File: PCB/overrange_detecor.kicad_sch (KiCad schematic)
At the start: 25 parts, among them Q301 DMP3125L, Q302 DMP3125L, U301 TLV3542, U302 74HC00, U303 LM321

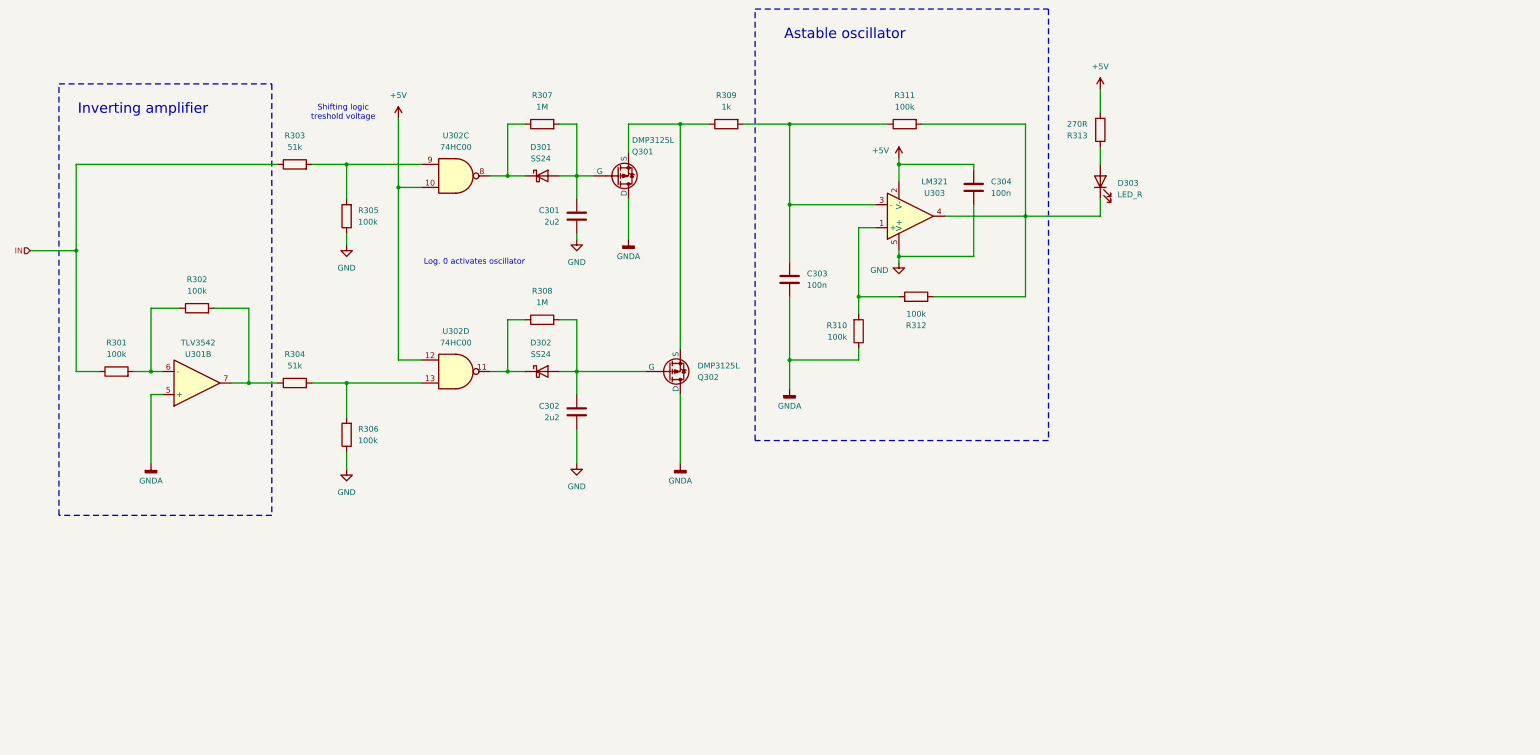
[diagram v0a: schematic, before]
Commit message: changes
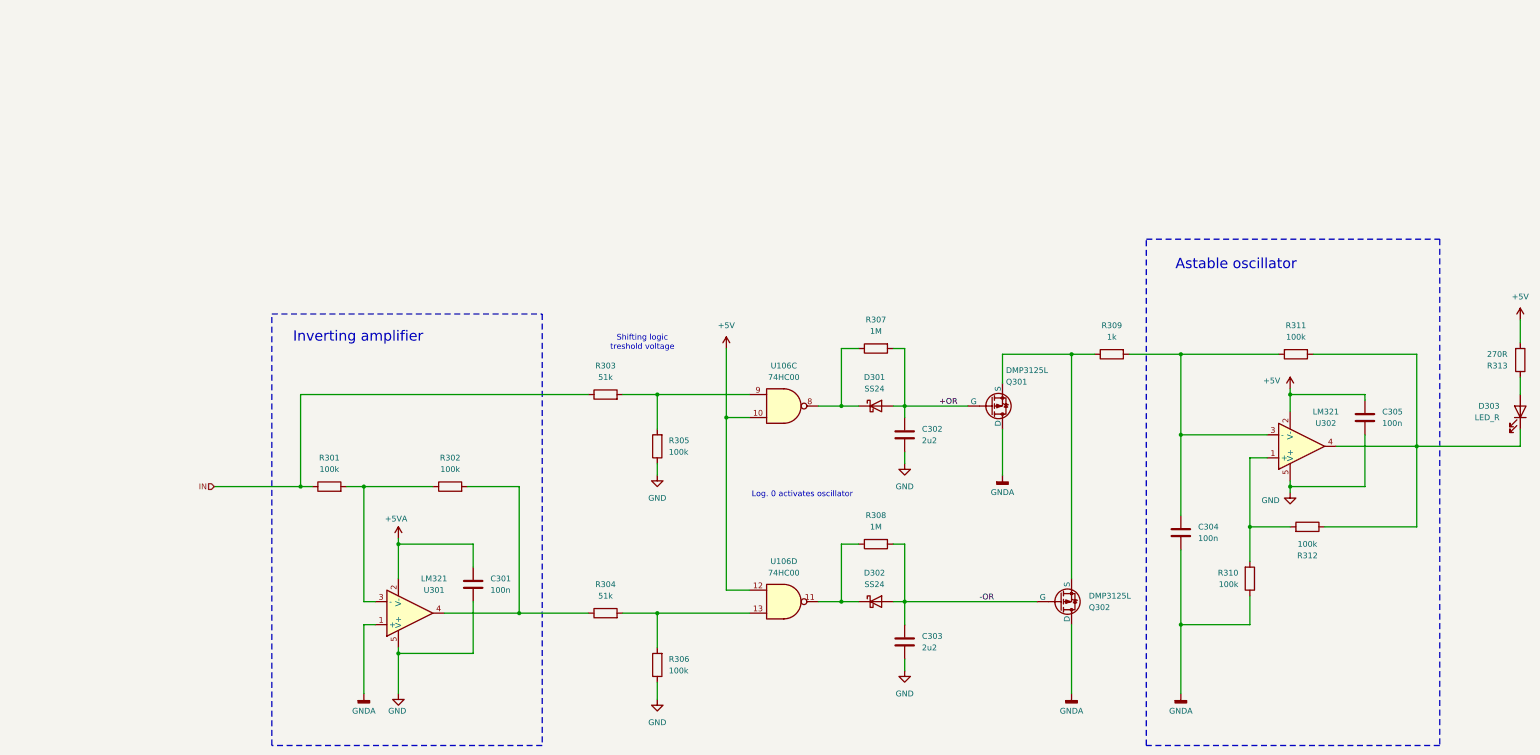
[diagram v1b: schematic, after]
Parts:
- removed U301: TLV3542, w-ic:SOIC-8, symbol w-analog-ic:TLV3542
- removed U302: 74HC00, w-ic:SOIC-14 208mil, symbol 74xx:74HC00
- added C303: 2u2, Capacitor_SMD:C_0603_1608Metric, symbol Device:C
- added U106: 74HC00, w-ic:SOIC-14 3.9x8.6mm P1.27mm, symbol 74xx:74HC00
- added U301: LM321, w-ic:SOT-23-5L, symbol w-analog-ic:LM321
- C301: value 2u2 -> 100n
- D301, D302: footprint Diode_SMD:D_SMA -> w-diode:SOD-123LF
- renumbered C303 to C304, C304 to C305, U303 to U302
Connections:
- net +5V: now also U106.10, U106.12
- net GND: now also C303.2, U301.5 (V+)
- net GNDA: now also U301.1 (+)
- net at D302.1 (K), R308.1: now also U106.11
- net -OR: now reaches D302.2 (A), Q302.1 (G), R308.2
- net -OR: now also C303.1; no longer C302.1
- net at R303.2, R305.2: now also U106.9
- net +OR: now reaches D301.2 (A), Q301.1 (G), R307.2
- net +OR: now also C302.1; no longer C301.1
- net at D301.1 (K), R307.1: now also U106.8
- net at R304.2, R306.2: now also U106.13
- net at R302.2, R304.1: now also U301.4
- net at R301.2, R302.1: now also U301.3 (-)
- new net +5VA: C301.1, U301.2 (V-)
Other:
- moved on the sheet: C304, C305, D303, Q301, Q302, R301, R302, R303, R304, R305, R306, R309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
